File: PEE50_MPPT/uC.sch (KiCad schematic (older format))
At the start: 3 parts, among them U4 MSP430FR2353TDBT

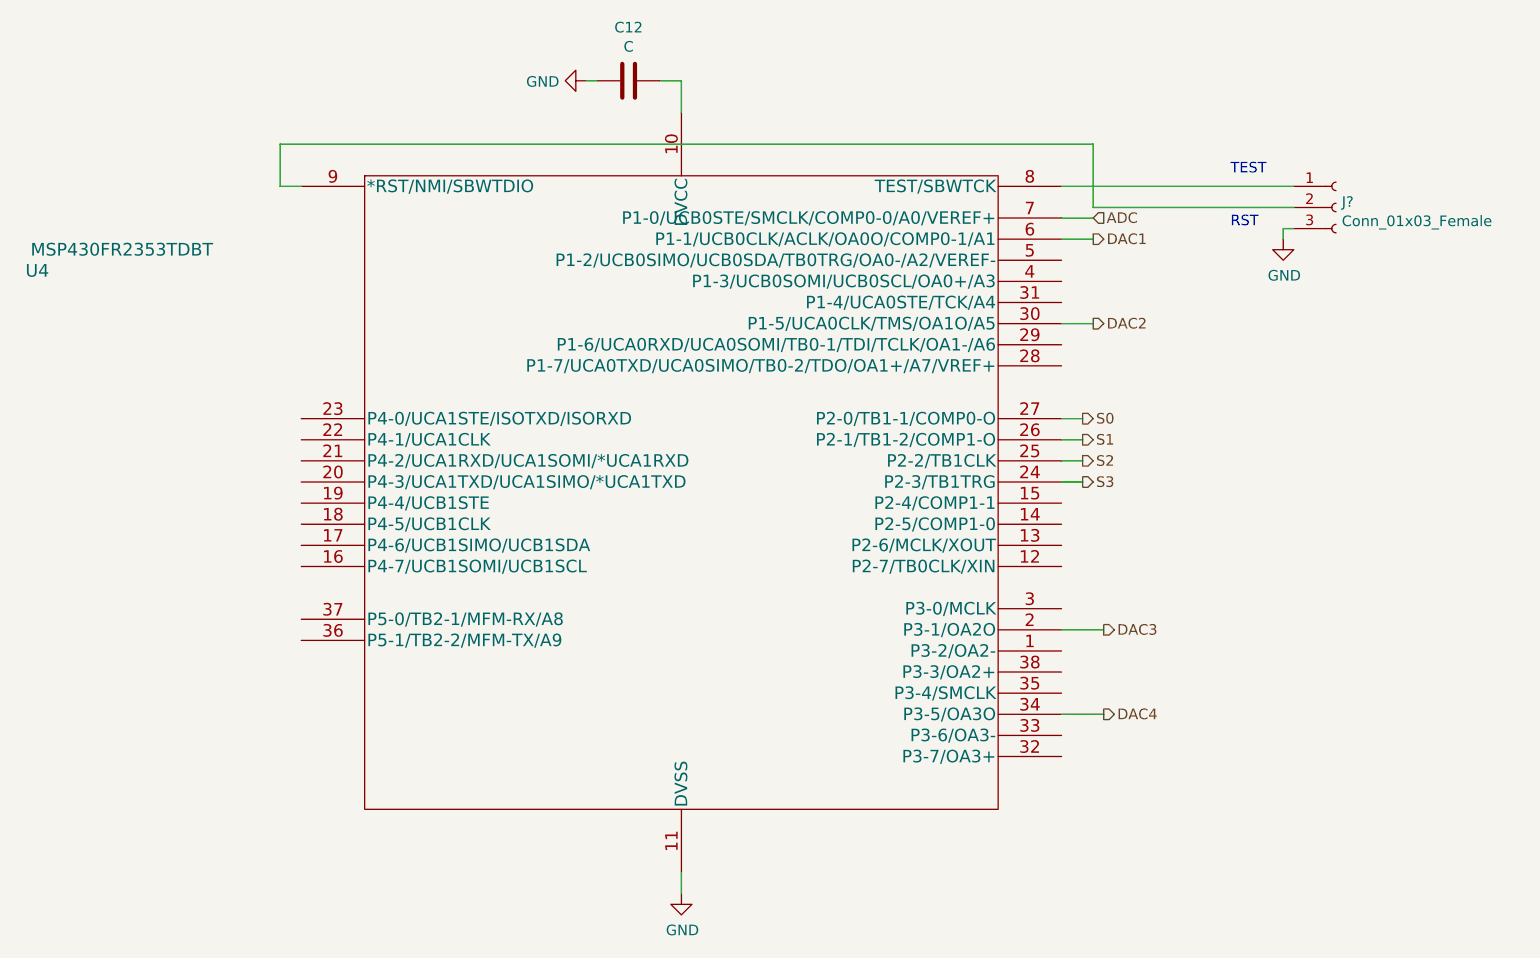
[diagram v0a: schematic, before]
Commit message: schakeling klaar (denk ik)
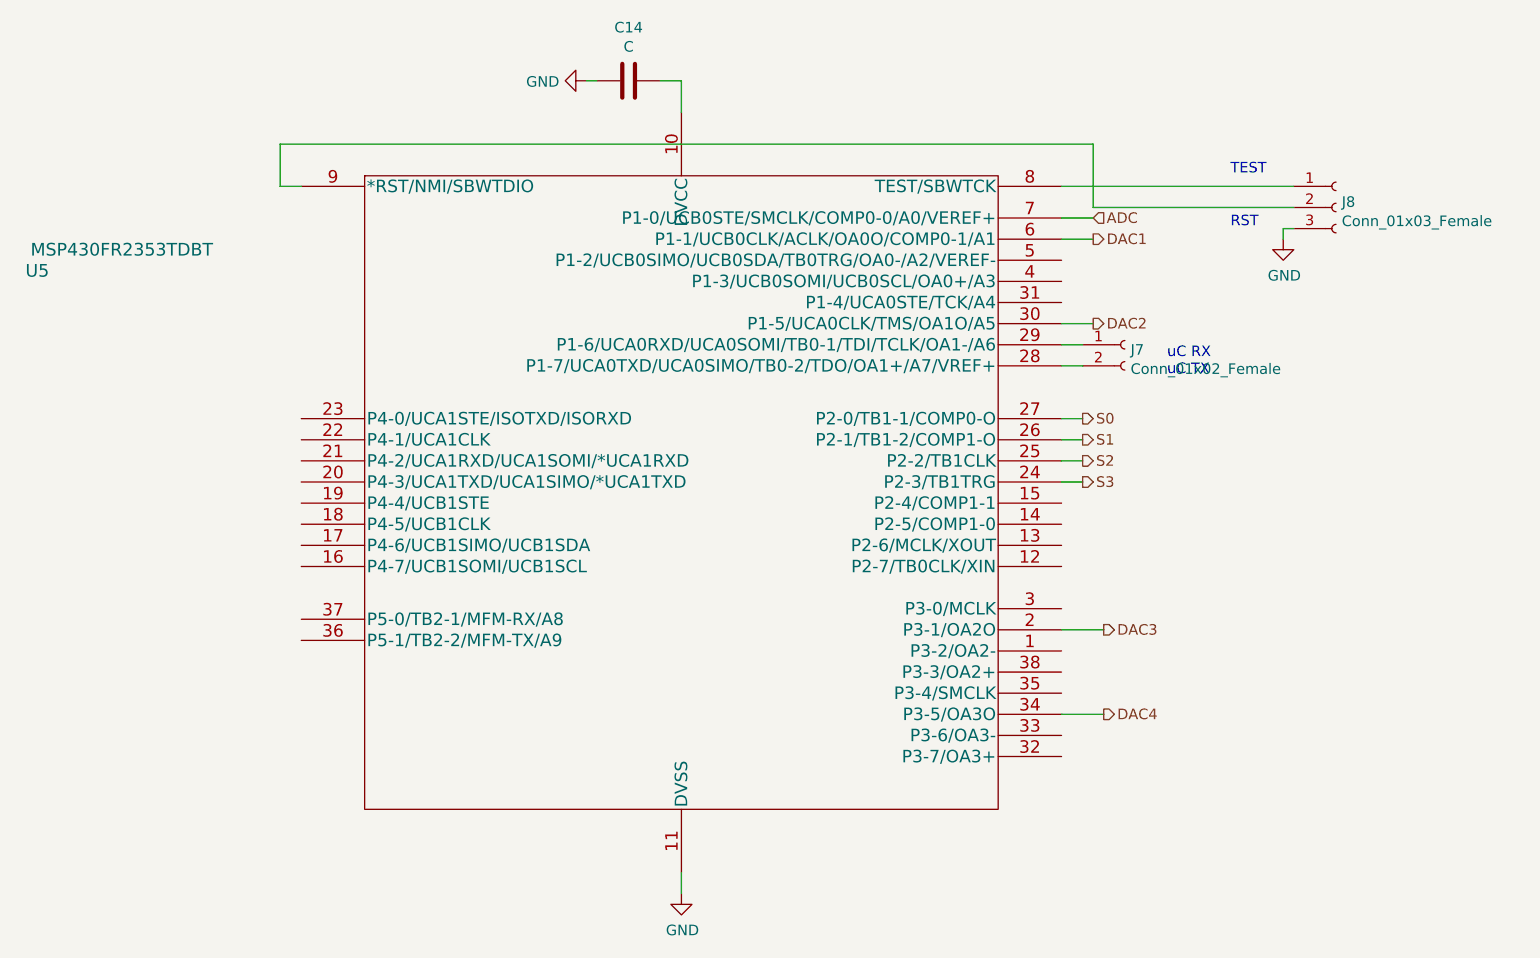
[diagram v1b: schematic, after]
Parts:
- added J7: Conn_01x02_Female, symbol Connector:Conn_01x02_Female
- gave numbers to parts that had none: 1
- renumbered C12 to C14, U4 to U5
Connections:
- net at U5.28 (P1-7/UCA0TXD/UCA0SIMO/TB0-2/TDO/OA1+/A7/VREF+): now also J7.2 (Pin_2)
- net at U5.29 (P1-6/UCA0RXD/UCA0SOMI/TB0-1/TDI/TCLK/OA1-/A6): now also J7.1 (Pin_1)
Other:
- note added: "uC RX\nuC TX\n"
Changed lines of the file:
@@
 $EndDescr
 $Comp
-L Robin_lib:MSP430FR2353TDBT U4
+L Robin_lib:MSP430FR2353TDBT U5
 U 1 1 608BCC4E
 P 5700 3600
-F 0 "U4" H 2650 4650 60  0000 C CNN
+F 0 "U5" H 2650 4650 60  0000 C CNN
 F 1 "MSP430FR2353TDBT" H 3050 4750 60  0000 C CNN
 F 2 "DBT38_TEX" H 4950 5250 60  0001 C CNN
@@
 $EndComp
 $Comp
-L power:GND #PWR0111
+L power:GND #PWR028
 U 1 1 608BCC99
 P 5700 5500
-F 0 "#PWR0111" H 5700 5250 50  0001 C CNN
+F 0 "#PWR028" H 5700 5250 50  0001 C CNN
 F 1 "GND" H 5705 5327 50  0000 C CNN
 F 2 "" H 5700 5500 50  0001 C CNN
@@
 	5700 5500 5700 5400
 $Comp
-L Device:C C12
+L Device:C C14
 U 1 1 608BF0BE
 P 5450 1650
-F 0 "C12" V 5198 1650 50  0000 C CNN
+F 0 "C14" V 5198 1650 50  0000 C CNN
 F 1 "C" V 5289 1650 50  0000 C CNN
 F 2 "" H 5488 1500 50  0001 C CNN
@@
 	5700 1650 5700 1800
 $Comp
-L power:GND #PWR0112
+L power:GND #PWR027
 U 1 1 608BF145
 P 5250 1650
-F 0 "#PWR0112" H 5250 1400 50  0001 C CNN
+F 0 "#PWR027" H 5250 1400 50  0001 C CNN
 F 1 "GND" V 5255 1522 50  0000 R CNN
 F 2 "" H 5250 1650 50  0001 C CNN
@@
 	7700 4650 7500 4650
 $Comp
-L Connector:Conn_01x03_Female J?
+L Connector:Conn_01x03_Female J8
 U 1 1 608C3F1C
 P 8800 2250
-F 0 "J?" H 8827 2276 50  0000 L CNN
+F 0 "J8" H 8827 2276 50  0000 L CNN
 F 1 "Conn_01x03_Female" H 8827 2185 50  0000 L CNN
 F 2 "" H 8800 2250 50  0001 C CNN
@@
 	3800 2150 3900 2150
 $Comp
-L power:GND #PWR0133
+L power:GND #PWR029
 U 1 1 608C4239
 P 8550 2400
-F 0 "#PWR0133" H 8550 2150 50  0001 C CNN
+F 0 "#PWR029" H 8550 2150 50  0001 C CNN
 F 1 "GND" H 8555 2227 50  0000 C CNN
 F 2 "" H 8550 2400 50  0001 C CNN
@@
 Wire Wire Line
 	7500 3250 7600 3250
+$Comp
+L Connector:Conn_01x02_Female J7
+U 1 1 6091D58E
+P 7800 2900
+F 0 "J7" H 7827 2876 50  0000 L CNN
+F 1 "Conn_01x02_Female" H 7827 2785 50  0000 L CNN
+F 2 "" H 7800 2900 50  0001 C CNN
+F 3 "~" H 7800 2900 50  0001 C CNN
+	1    7800 2900
+	1    0    0    -1
+$EndComp
+Wire Wire Line
+	7500 2900 7600 2900
+Wire Wire Line
+	7500 3000 7600 3000
+Text Notes 8000 3050 0    50   ~ 0
+uC RX\nuC TX\n
 $EndSCHEMATC
